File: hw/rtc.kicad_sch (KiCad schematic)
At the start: 6 parts, among them U9 BQ32002DR

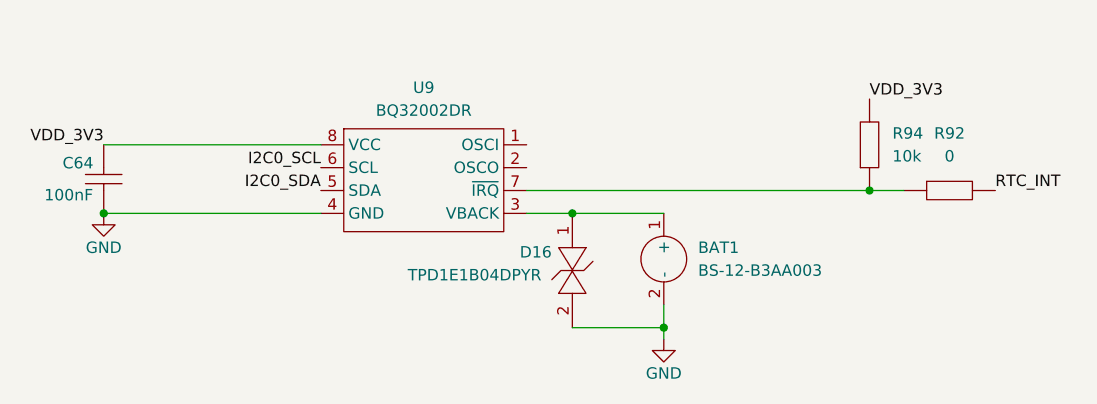
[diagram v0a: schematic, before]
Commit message: eMMC draft
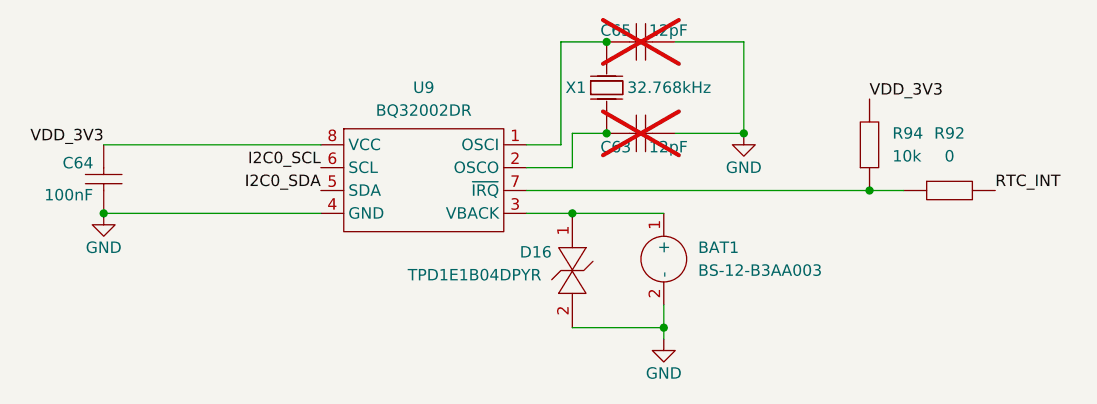
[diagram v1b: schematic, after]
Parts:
- added C63, C65: C0805C120J5GACAUTO, pepy_sym_lib:[CAP_SMD_0805_2012Metric], symbol pepy_sym_lib:[CAP_SMD_0805_2012Metric]KEMET C0805C120J5GACAUTO
- added X1: SC-20S32.768kHz20PPM9pF, pepy_sym_lib:[Crystal_32_768_kHZ]Seiko SC-20S,32.768kHz,20PPM,9pF, symbol pepy_sym_lib:[Crystal_32_768_kHZ]Seiko SC-20S,32.768kHz,20PPM,9pF
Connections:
- net GND: now also C63.1, C65.1
- net at U9.1 (OSCI): now also C65.2, X1.1
- net at U9.2 (OSCO): now also C63.2, X1.2

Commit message: WIP SIM module
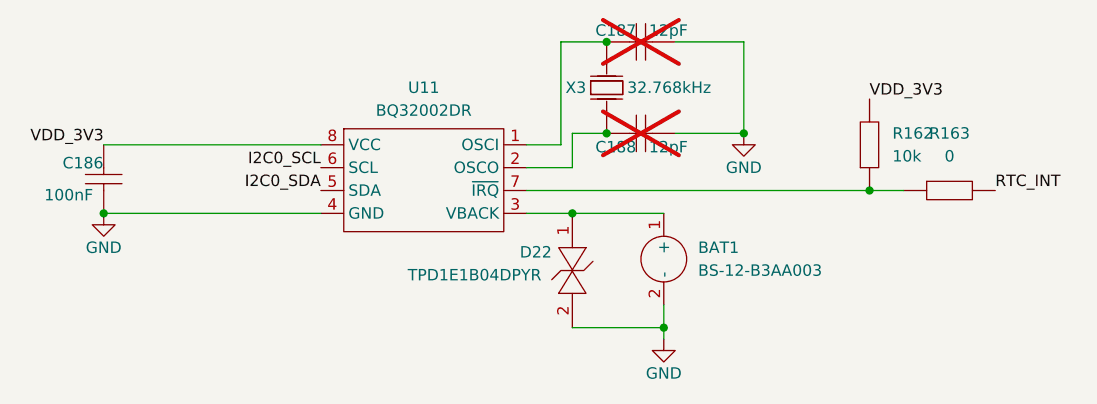
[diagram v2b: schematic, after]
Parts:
- renumbered C64 to C186, C65 to C187, C63 to C188, D16 to D22, R94 to R162, R92 to R163, U9 to U11, X1 to X3
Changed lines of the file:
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@@
 		(on_board yes)
 		(dnp no)
-		(property "Reference" "#PWR068"
+		(property "Reference" "#PWR0123"
 			(at 125.73 77.47 0)
 			(effects
@@
 			(project "dashcam"
 				(path "/30d6913c-7aa4-4f56-9882-2ba08f7e2cce/d699a9f8-e4b6-41ca-8e95-ac75f365d4d0"
-					(reference "#PWR068")
+					(reference "#PWR0123")
 					(unit 1)
 				)
@@
 		(on_board yes)
 		(dnp no)
-		(property "Reference" "#PWR067"
+		(property "Reference" "#PWR0122"
 			(at 116.84 100.33 0)
 			(effects
@@
 			(project "dashcam"
 				(path "/30d6913c-7aa4-4f56-9882-2ba08f7e2cce/d699a9f8-e4b6-41ca-8e95-ac75f365d4d0"
-					(reference "#PWR067")
+					(reference "#PWR0122")
 					(unit 1)
 				)
@@
 		(on_board yes)
 		(dnp no)
-		(property "Reference" "D16"
+		(property "Reference" "D22"
 			(at 100.838 84.328 90)
 			(effects
@@
 			(project ""
 				(path "/30d6913c-7aa4-4f56-9882-2ba08f7e2cce/d699a9f8-e4b6-41ca-8e95-ac75f365d4d0"
-					(reference "D16")
+					(reference "D22")
 					(unit 1)
 				)
@@
 		(on_board yes)
 		(dnp no)
-		(property "Reference" "#PWR066"
+		(property "Reference" "#PWR0121"
 			(at 54.61 86.36 0)
 			(effects
@@
 			(project ""
 				(path "/30d6913c-7aa4-4f56-9882-2ba08f7e2cce/d699a9f8-e4b6-41ca-8e95-ac75f365d4d0"
-					(reference "#PWR066")
+					(reference "#PWR0121")
 					(unit 1)
 				)
@@
 		(dnp no)
 		(fields_autoplaced yes)
-		(property "Reference" "U9"
+		(property "Reference" "U11"
 			(at 90.17 66.04 0)
 			(effects
@@
 			(project ""
 				(path "/30d6913c-7aa4-4f56-9882-2ba08f7e2cce/d699a9f8-e4b6-41ca-8e95-ac75f365d4d0"
-					(reference "U9")
+					(reference "U11")
 					(unit 1)
 				)
@@
 		(on_board yes)
 		(dnp no)
-		(property "Reference" "C64"
+		(property "Reference" "C186"
 			(at 50.038 74.422 90)
 			(effects
@@
 			(project ""
 				(path "/30d6913c-7aa4-4f56-9882-2ba08f7e2cce/d699a9f8-e4b6-41ca-8e95-ac75f365d4d0"
-					(reference "C64")
+					(reference "C186")
 					(unit 1)
 				)
@@
 		(dnp no)
 		(fields_autoplaced yes)
-		(property "Reference" "R92"
+		(property "Reference" "R163"
 			(at 148.59 71.12 0)
 			(effects
@@
 			(project ""
 				(path "/30d6913c-7aa4-4f56-9882-2ba08f7e2cce/d699a9f8-e4b6-41ca-8e95-ac75f365d4d0"
-					(reference "R92")
+					(reference "R163")
 					(unit 1)
 				)
@@
 		(on_board yes)
 		(dnp no)
-		(property "Reference" "X1"
+		(property "Reference" "X3"
 			(at 105.918 66.04 90)
 			(effects
@@
 			(project ""
 				(path "/30d6913c-7aa4-4f56-9882-2ba08f7e2cce/d699a9f8-e4b6-41ca-8e95-ac75f365d4d0"
-					(reference "X1")
+					(reference "X3")
 					(unit 1)
 				)
@@
 		(dnp no)
 		(fields_autoplaced yes)
-		(property "Reference" "R94"
+		(property "Reference" "R162"
 			(at 142.24 71.1199 90)
 			(effects
@@
 			(project ""
 				(path "/30d6913c-7aa4-4f56-9882-2ba08f7e2cce/d699a9f8-e4b6-41ca-8e95-ac75f365d4d0"
-					(reference "R94")
+					(reference "R162")
 					(unit 1)
 				)
@@
 		(on_board yes)
 		(dnp yes)
-		(property "Reference" "C63"
+		(property "Reference" "C188"
 			(at 111.506 72.644 0)
 			(effects
@@
 			(project ""
 				(path "/30d6913c-7aa4-4f56-9882-2ba08f7e2cce/d699a9f8-e4b6-41ca-8e95-ac75f365d4d0"
-					(reference "C63")
+					(reference "C188")
 					(unit 1)
 				)
@@
 		(on_board yes)
 		(dnp yes)
-		(property "Reference" "C65"
+		(property "Reference" "C187"
 			(at 111.506 59.69 0)
 			(effects
@@
 			(project "dashcam"
 				(path "/30d6913c-7aa4-4f56-9882-2ba08f7e2cce/d699a9f8-e4b6-41ca-8e95-ac75f365d4d0"
-					(reference "C65")
-					(unit 1)
-				)
+					(reference "C187")
+					(unit 1)
+				)
